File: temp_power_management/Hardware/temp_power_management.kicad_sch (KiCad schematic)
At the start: 43 parts, among them J1 BAT1_IN, J10 CAN, J11 Conn_01x08_Pin, J12 5V Converter IN, J13 5V Converter OUT, J2 BAT_OUT1, J3 BAT2_IN, J4 BAT_OUT2, J5 BAT_OUT3, J6 BAT_OUT4, J7 BAT_OUT5, J8 BAT_OUT5, J9 CHG_PORT, K1 RELPOL R40N-3021-85-1024, Q1 SIDR392DP-T1-GE3, SW1 SW_Push, SW2 EMERG_STOP, U1 STM32F103CBTx, U2 NCP114BSN330T1G

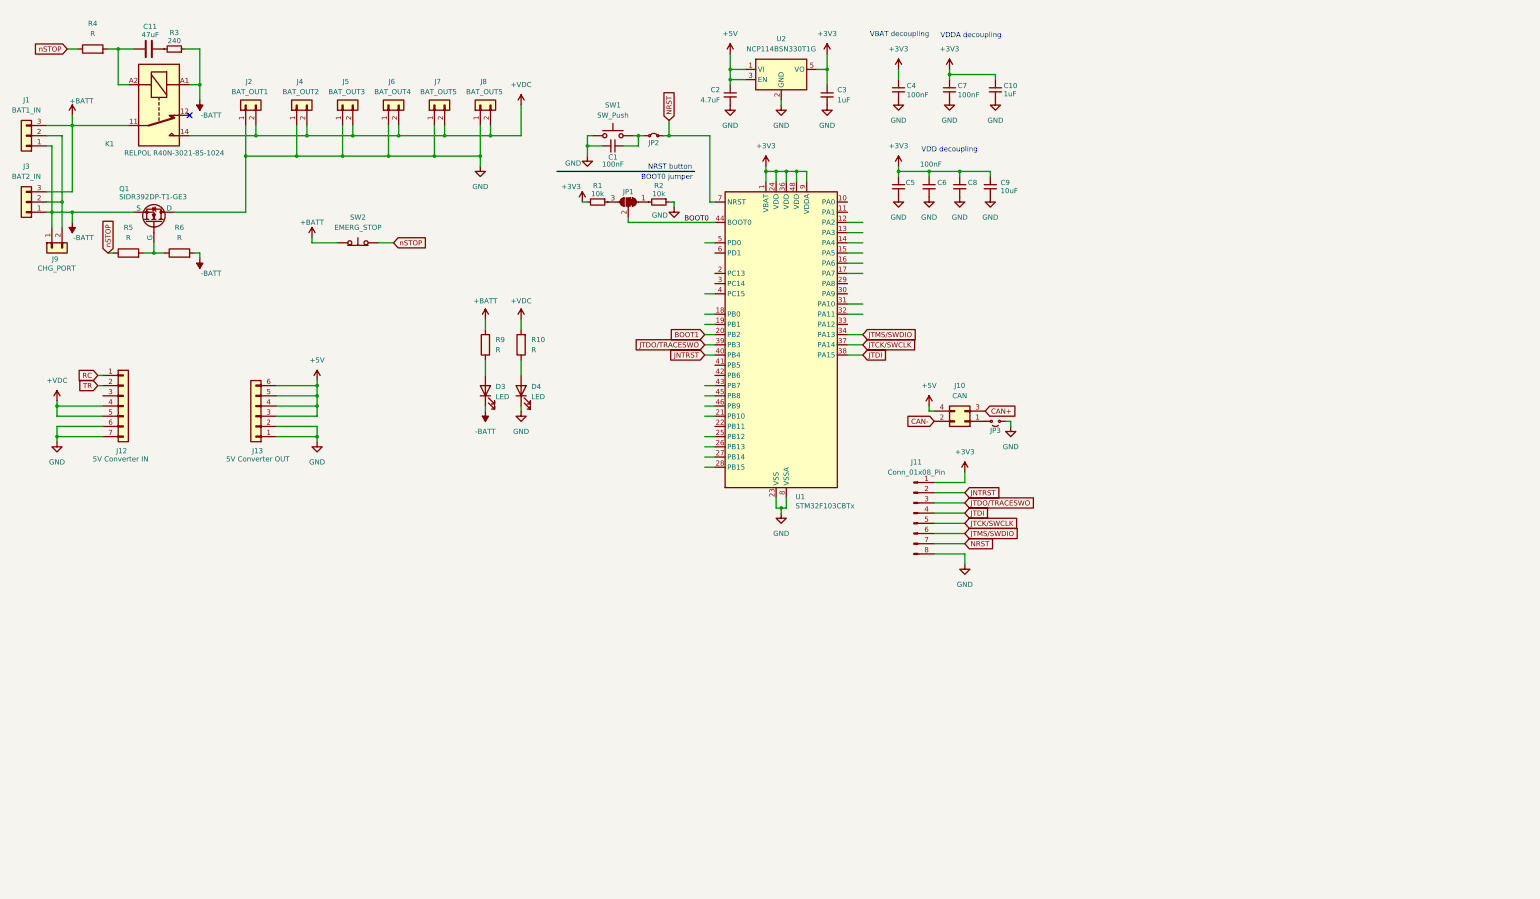
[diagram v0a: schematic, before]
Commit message: temp_PMS - much done, kill me
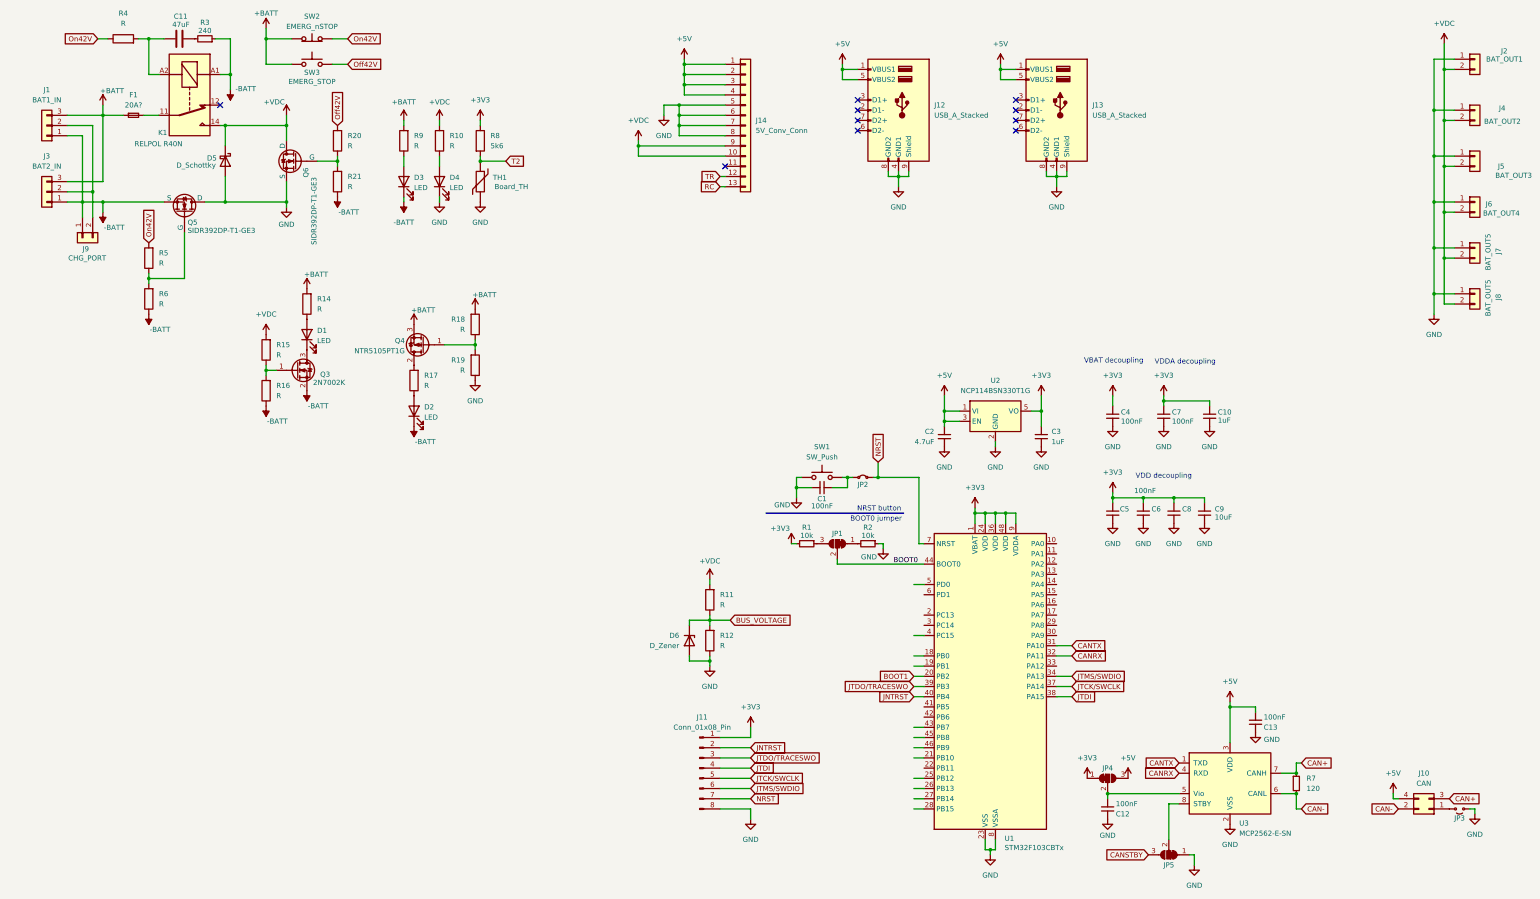
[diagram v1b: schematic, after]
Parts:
- removed J12: 5V Converter IN, symbol Connector_Generic:Conn_01x07
- removed J13: 5V Converter OUT, symbol Connector_Generic:Conn_01x06
- removed Q1: SIDR392DP-T1-GE3, firo_footprints:PowerPAK_SO-8DC for VISHAY SIDR392DP-T1-GE3, symbol Simulation_SPICE:NMOS
- added C12, C13: 100nF, Capacitor_SMD:C_0402_1005Metric, symbol Device:C_Small
- added D1, D2: LED, symbol Device:LED
- added D5: D_Schottky, symbol Device:D_Schottky
- added D6: D_Zener, symbol Device:D_Zener
- added F1: 20A?, symbol Device:Fuse_Small
- added J12, J13: USB_A_Stacked, Connector_USB:USB_A_CUI_UJ2-ADH-TH_Horizontal_Stacked, symbol Connector:USB_A_Stacked
- added J14: 5V_Conv_Conn, firo_footprints:MeanWell NID100-R3, symbol Connector_Generic:Conn_01x13
- added JP4, JP5: SolderJumper_3_Bridged12, Jumper:SolderJumper-3_P1.3mm_Bridged12_RoundedPad1.0x1.5mm, symbol Jumper:SolderJumper_3_Bridged12
- added Q3: 2N7002K, Package_TO_SOT_SMD:SOT-23, symbol Transistor_FET:2N7002K
- added Q4: NTR5105PT1G, Package_TO_SOT_SMD:SOT-223-3_TabPin2, symbol Device:Q_PMOS_GDS
- added Q5, Q6: SIDR392DP-T1-GE3, firo_footprints:PowerPAK_SO-8DC for VISHAY SIDR392DP-T1-GE3, symbol Simulation_SPICE:NMOS
- added R11, R12, R14, R15, R16, R17, R18, R19, R20, R21: R, symbol Device:R
- added R7: 120, Resistor_SMD:R_0805_2012Metric, symbol Device:R_Small
- added R8: 5k6, Resistor_SMD:R_0402_1005Metric, symbol Device:R
- added SW3: EMERG_STOP, Button_Switch_SMD:SW_SPST_EVQP7C, symbol Switch:SW_Push
- added TH1: Board_TH, Resistor_SMD:R_0603_1608Metric, symbol Device:Thermistor
- added U3: MCP2562-E-SN, Package_SO:SOIC-8_3.9x4.9mm_P1.27mm, symbol Interface_CAN_LIN:MCP2562-E-SN
- K1: value RELPOL R40N-3021-85-1024 -> RELPOL R40N
- SW2: value EMERG_STOP -> EMERG_nSTOP
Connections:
- net +3V3: now also JP4.1 (A), R8.1
- net +5V: now also C13.2, J12.1 (VBUS1), J12.5 (VBUS2), J13.1 (VBUS1), J13.5 (VBUS2), J14.1 (Pin_1), J14.2 (Pin_2), J14.3 (Pin_3), J14.4 (Pin_4), JP4.3 (B), U3.3 (VDD)
- net +BATT: now also F1.1, Q4.3 (S), R14.2, R18.2, SW3.1; no longer K1.11
- net +VDC: now also D5.1 (K), J14.10 (Pin_10), J14.9 (Pin_9), Q6.3 (D), R11.2, R15.2
- net -BATT: now also R6.1, D2.1 (K), Q3.2 (S), Q5.1 (S), R16.1, R21.1; no longer R6.2
- net CAN+: now also R7.1, U3.7 (CANH)
- net CAN-: now also R7.2, U3.6 (CANL)
- net GND: now also C12.1, C13.1, D5.2 (A), D6.2 (A), J12.4 (GND1), J12.8 (GND2), J12.9 (Shield), J13.4 (GND1), J13.8 (GND2), J13.9 (Shield), J14.5 (Pin_5), J14.6 (Pin_6), J14.7 (Pin_7), J14.8 (Pin_8), JP5.1 (A), Q5.3 (D), Q6.1 (S), R12.1, R19.1, TH1.2, U3.2 (VSS)
- net RC: now also J14.13 (Pin_13)
- net TR: now also J14.12 (Pin_12)
- net On42V: now reaches R5.2
- net On42V: now also R4.1, SW2.2 (B); no longer R6.1
- net CANTX: now reaches U1.31 (PA10)
- net CANTX: now also U3.1 (TXD)
- net CANRX: now reaches U1.32 (PA11)
- net CANRX: now also U3.4 (RXD)
- removed net nSTOP: R4.1, R5.1, SW2.2 (B)
- new net: C12.2, JP4.2 (C), U3.5 (Vio)
- new net: D2.2 (A), R17.1
- new net: Q3.1 (G), R15.1, R16.2
- new net: Q6.2 (G), R20.1, R21.2
- new net: Q4.1 (G), R18.1, R19.2
- new net: D1.1 (K), Q3.3 (D)
- new net: D1.2 (A), R14.1
- new net: JP5.2 (C), U3.8 (STBY)
- new net: Q5.2 (G), R5.1, R6.2
- new net: F1.2, K1.11
- new net: Q4.2 (D), R17.2
- new net BUS_VOLTAGE: D6.1 (K), R11.1, R12.2
- new net CANSTBY: JP5.3 (B)
- new net Off42V: R20.2, SW3.2
- new net T2: R8.2, TH1.1
- no-connect marks 1 -> 10
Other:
- moved on the sheet: C1, C10, C11, C2, C3, C4, C5, C6, C7, C8, C9, D3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
